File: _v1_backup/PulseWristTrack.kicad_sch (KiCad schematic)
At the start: 16 parts, among them J1 BATT_JST_PH, Q1 BSS138, Q2 BSS138, SW1 JS102011SAQN, U1 XIAO_nRF52840_Sense, U2 MAX30102, U3 AP2112K-1.8

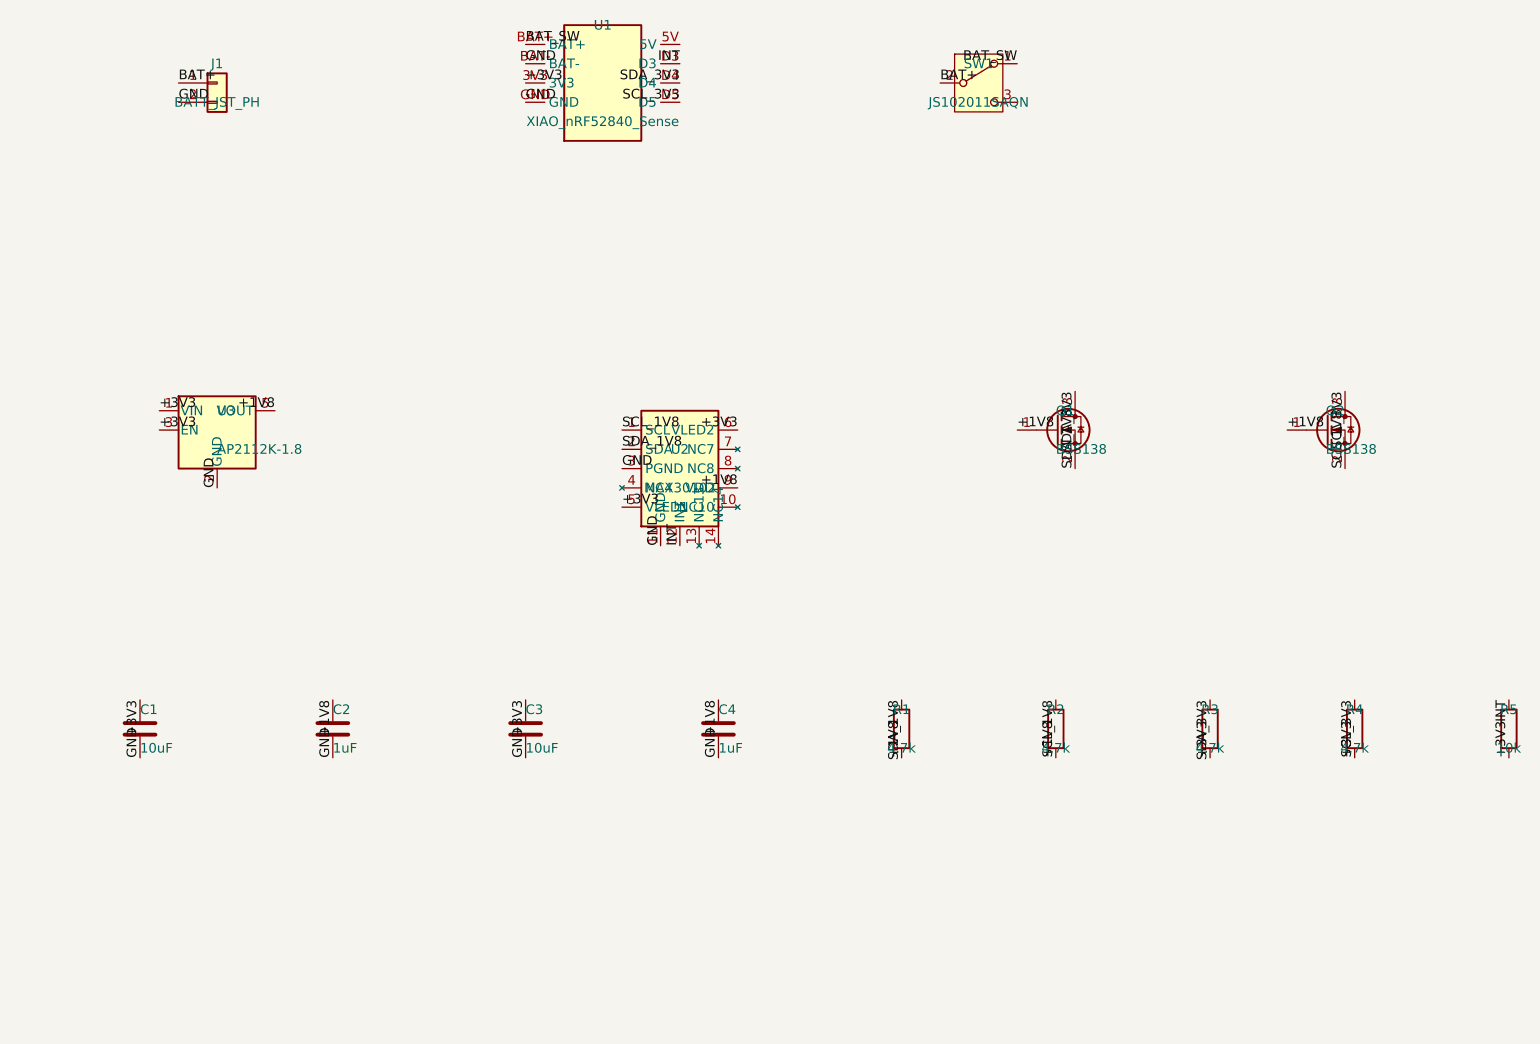
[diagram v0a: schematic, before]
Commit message: auto-backup 2026-07-24 19:26:27
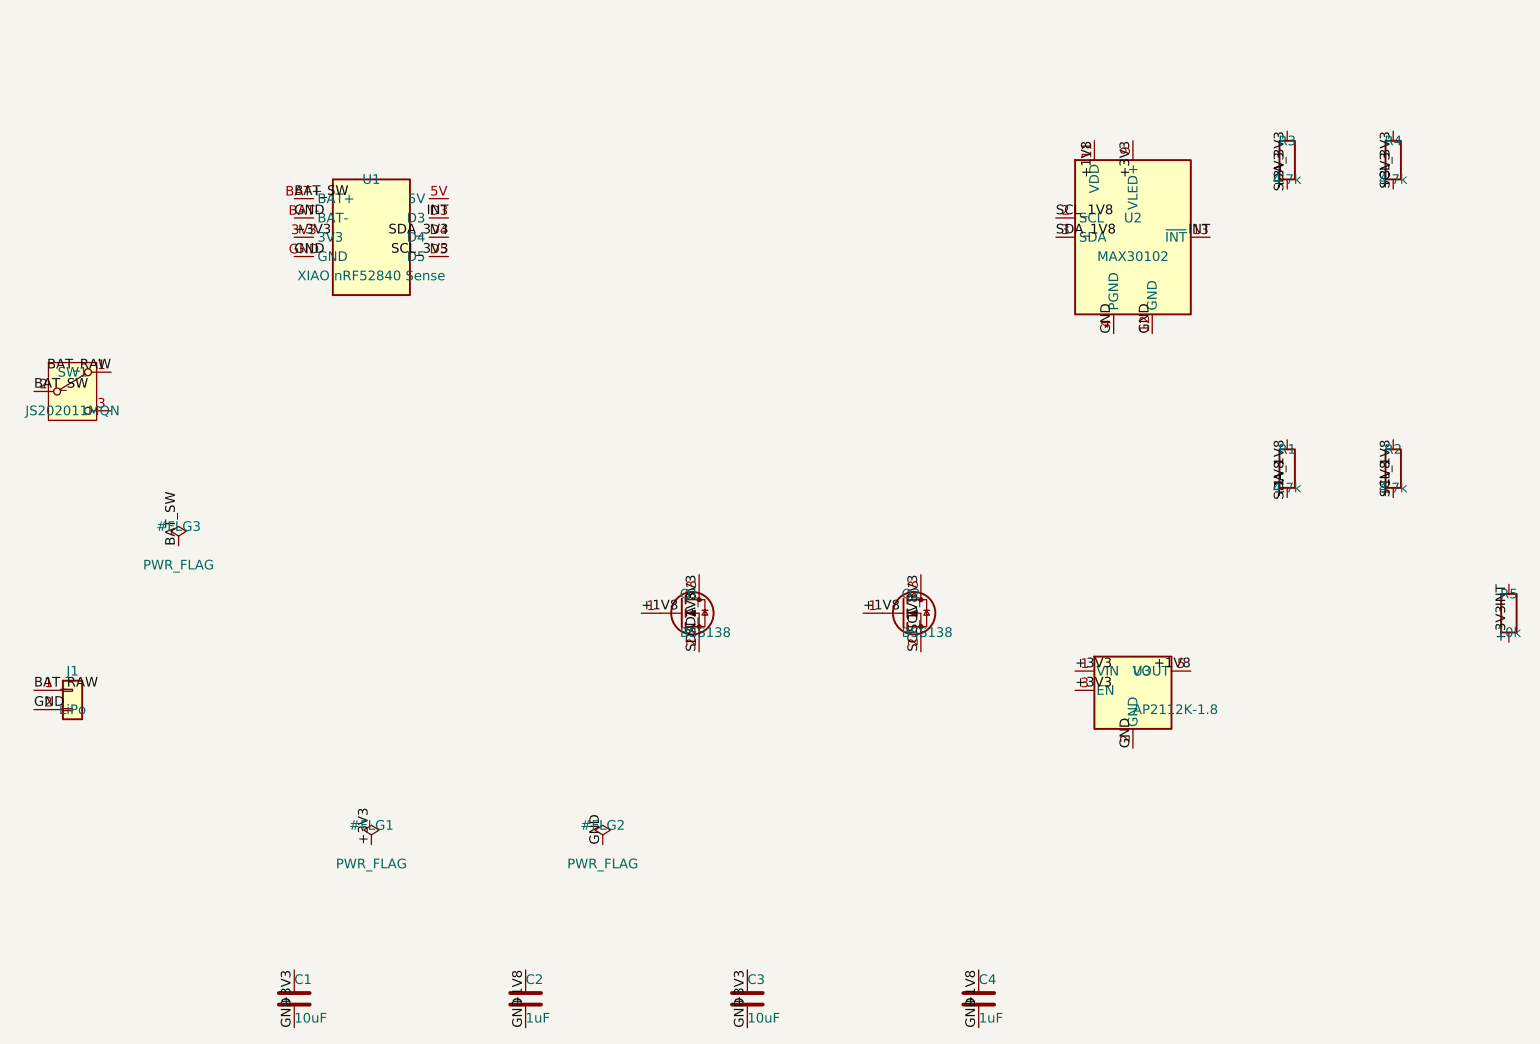
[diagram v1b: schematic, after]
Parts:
- removed U2: MAX30102, PulseWristTrack:MAX30102_OLGA14, symbol PulseWristTrack:MAX30102
- added U2: MAX30102, PulseWristTrack:MAX30102_OLGA14, symbol Sensor:MAX30102
- J1: value BATT_JST_PH -> LiPo
- SW1: value JS102011SAQN -> JS202011MQN; footprint Button_Switch_SMD:SW_SPDT_CK_JS102011SAQN -> Button_Switch_SMD:SW_SPDT_PCM12
- U1: value XIAO_nRF52840_Sense -> XIAO nRF52840 Sense
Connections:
- net +1V8: now also U2.11 (VDD)
- net +3V3: now also U2.10 (VLED+), U2.9 (VLED+)
- net BAT_SW: now also SW1.2 (B); no longer SW1.1 (A)
- net GND: now also U2.12 (GND), U2.4 (PGND)
- net INT: now also U2.13 (~{INT})
- net SCL_1V8: now also U2.2 (SCL)
- net SDA_1V8: now also U2.3 (SDA)
- net BAT+ renamed BAT_RAW
- net BAT_RAW: now also SW1.1 (A); no longer SW1.2 (B)
